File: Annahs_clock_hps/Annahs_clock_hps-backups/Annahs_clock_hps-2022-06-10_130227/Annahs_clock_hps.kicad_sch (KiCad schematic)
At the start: 11 parts, among them SW1 Omron_B3F_SPST, SW2 Omron_B3F_SPST, SW3 Omron_B3F_SPST, SW4 Omron_B3F_SPST, U1 DS1307_DIP-8, U2 MAX7219

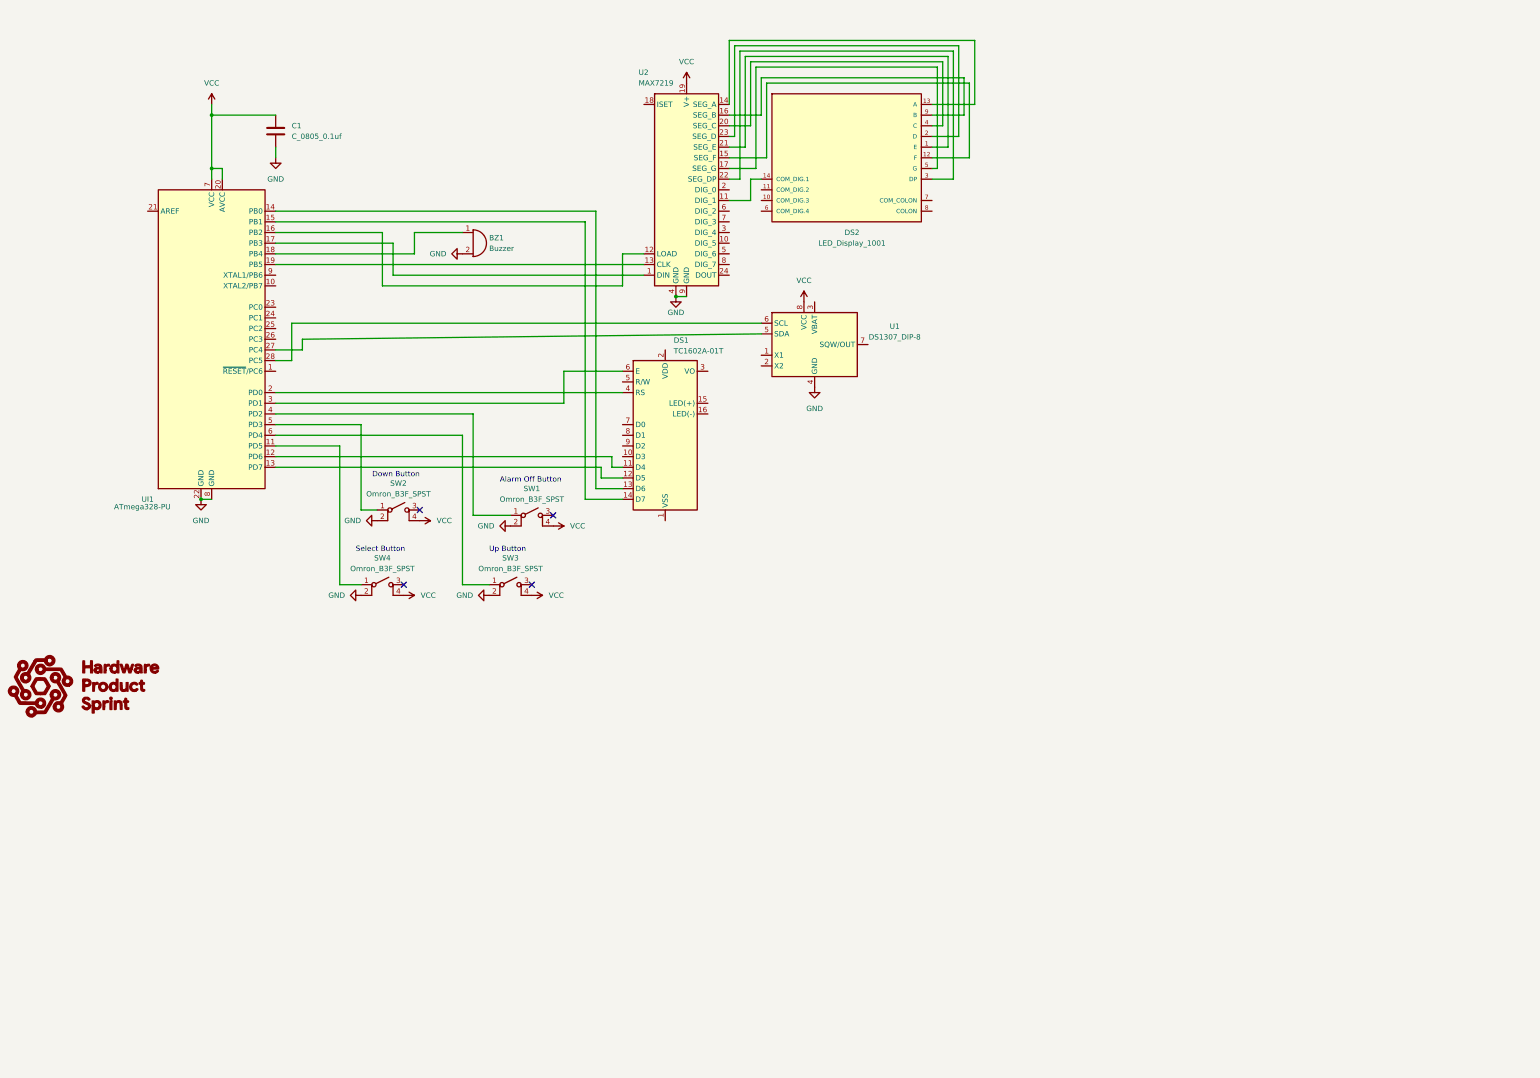
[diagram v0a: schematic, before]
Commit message: Update_Schematic
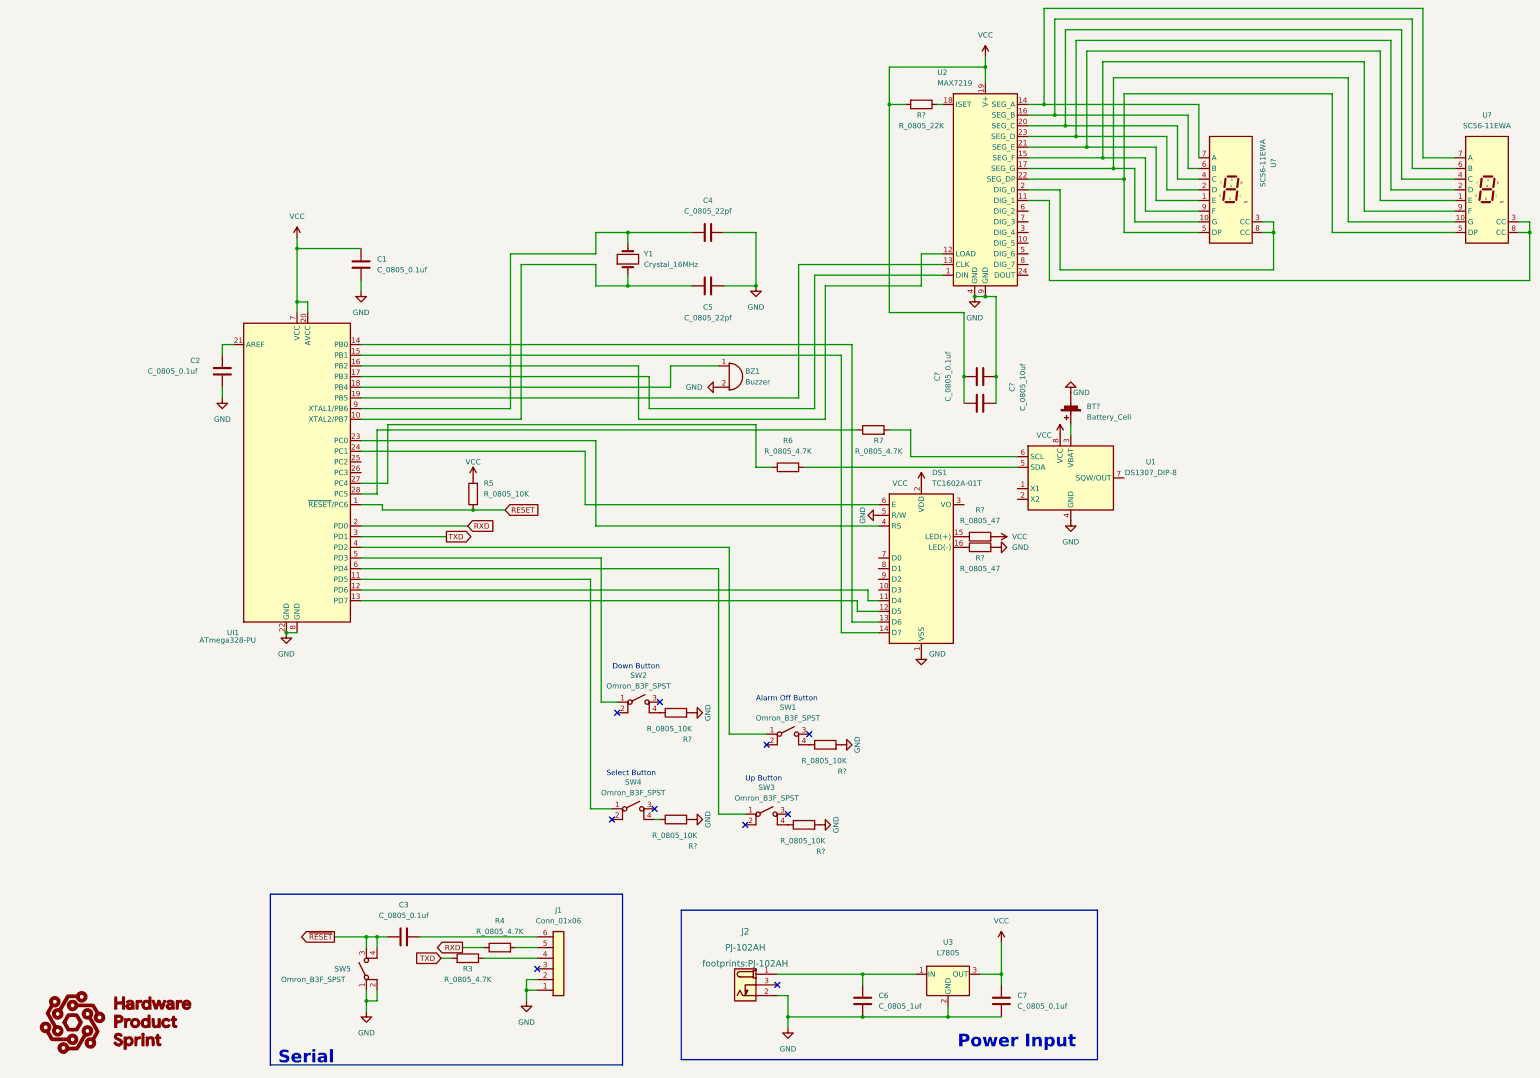
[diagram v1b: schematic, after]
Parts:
- removed DS2: LED_Display_1001, footprints:Adafruit-1001-0-0-MFG, symbol HPS:LED_Display_1001
- added BT?: Battery_Cell, footprints:BatteryHolder_Keystone_106_1x20mm, symbol HPS:Battery_Cell
- added C2, C3, C7, C?: C_0805_0.1uf, footprints:C_0805_2012Metric, symbol HPS:C_0805_0.1uf
- added C4, C5: C_0805_22pf, footprints:C_0805_2012Metric, symbol HPS:C_0805_22pf
- added C6: C_0805_1uf, footprints:C_0805_2012Metric, symbol HPS:C_0805_1uf
- added C?: C_0805_10uf, footprints:C_0805_2012Metric, symbol HPS:C_0805_10uf
- added J1: Conn_01x06, footprints:PinHeader_1x06_P2.54mm_Vertical, symbol HPS:Conn_01x06
- added J2: PJ-102AH, footprints:PJ-102AH, symbol HPS:PJ-102AH
- added R3, R4, R6, R7: R_0805_4.7K, footprints:R_0805_2012Metric, symbol HPS:R_0805_4.7K
- added R5, R? (x4): R_0805_10K, footprints:R_0805_2012Metric, symbol HPS:R_0805_10K
- added R?: R_0805_22K, footprints:R_0805_2012Metric, symbol HPS:R_0805_22K
- added R? (x2): R_0805_47, footprints:R_0805_2012Metric, symbol HPS:R_0805_47
- added SW5: Omron_B3F_SPST, footprints:SW_SPST_Omron_B3FS-100xP, symbol HPS:Omron_B3F_SPST
- added U3: L7805, symbol HPS_2:L7805
- added U? (x2): SC56-11EWA, Display_7Segment:Sx56-1xxxxx, symbol HPS:SC56-11EWA
- added Y1: Crystal_16MHz, footprints:Crystal_SMD_HC49-SD, symbol HPS:Crystal_16MHz
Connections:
- net GND: now also DS1.1 (VSS), DS1.5 (R/W), BT?.2 (-), C2.2, C4.1, C5.2, C6.2, C7.2, C?.2, C?.2, J1.1 (Pin_1), J1.2 (Pin_2), J2.2 (OUT), R?.2, R?.2, R?.2, R?.2, R?.2, SW5.1 (A), SW5.2 (A), U3.2 (GND); no longer SW1.2 (A), SW2.2 (A), SW3.2 (A), SW4.2 (A)
- net VCC: now also DS1.2 (VDD), C7.1, C?.1, C?.1, R5.2, R?.2, R?.2, U3.3 (OUT); no longer SW1.4 (B), SW2.4 (B), SW3.4 (B), SW4.4 (B)
- net at U1.3 (VBAT): now also BT?.1 (+)
- net at U1.5 (SDA): now also R6.2; no longer UI1.27 (PC4)
- net at U1.6 (SCL): now also R7.2; no longer UI1.28 (PC5)
- net at U2.21 (SEG_E): now also U?.1 (E), U?.1 (E)
- net at U2.15 (SEG_F): now also U?.9 (F), U?.9 (F)
- net at U2.14 (SEG_A): now also U?.7 (A), U?.7 (A)
- net at U2.11 (DIG_1): now also U?.3 (CC), U?.8 (CC)
- net at U2.23 (SEG_D): now also U?.2 (D), U?.2 (D)
- net at U2.22 (SEG_DP): now also U?.5 (DP), U?.5 (DP)
- net at U2.20 (SEG_C): now also U?.4 (C), U?.4 (C)
- net at U2.17 (SEG_G): now also U?.10 (G), U?.10 (G)
- net at U2.16 (SEG_B): now also U?.6 (B), U?.6 (B)
- net at U2.18 (ISET): now also R?.1
- net at U2.2 (DIG_0): now also U?.3 (CC), U?.8 (CC)
- net at DS1.15 (LED(+)): now also R?.1
- net at DS1.16 (LED(-)): now also R?.1
- net at DS1.4 (RS): now also UI1.23 (PC0); no longer UI1.2 (PD0)
- net at DS1.6 (E): now also UI1.24 (PC1); no longer UI1.3 (PD1)
- net RESET: now reaches UI1.1 (~{RESET}/PC6)
- net RESET: now also R5.1
- net at UI1.10 (XTAL2/PB7): now also C5.1, Y1.1
- net at UI1.21 (AREF): now also C2.1
- net at UI1.9 (XTAL1/PB6): now also C4.2, Y1.2
- new net: R?.1, SW2.4 (B)
- new net: J1.5 (Pin_5), R4.2
- new net: R?.1, SW3.4 (B)
- new net: R?.1, SW1.4 (B)
- new net: J1.4 (Pin_4), R3.1
- new net: C3.2, J1.6 (Pin_6)
- new net: R?.1, SW4.4 (B)
- new net: C6.1, J2.1 (POLE), U3.1 (IN)
- new net: R7.1, UI1.28 (PC5)
- new net: R6.1, UI1.27 (PC4)
- new net RXD: R4.1, UI1.2 (PD0)
- new net TXD: R3.2, UI1.3 (PD1)
- new net ~{RESET}: C3.1, SW5.3 (B), SW5.4 (B)
- no-connect marks 4 -> 10
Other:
- note added: "Power Input"
- note added: "Serial"
- moved on the sheet: BZ1, C1, DS1, SW1, SW2, SW3, SW4, U1, U2, UI1
